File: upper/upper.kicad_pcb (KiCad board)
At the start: 2 copper layers, 127 x 50.8 mm, 1 part, among them U1 RaspberryPi_Pico_W

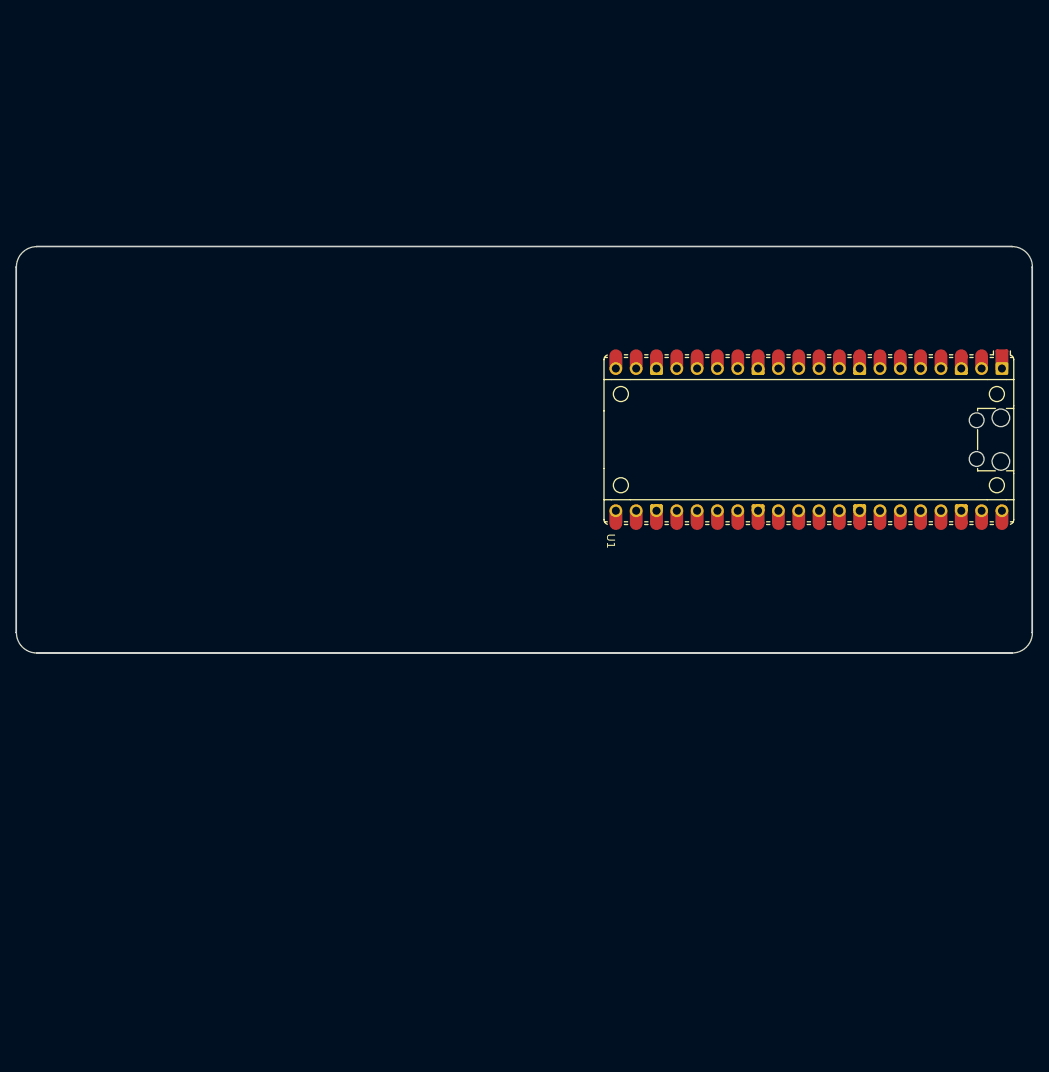
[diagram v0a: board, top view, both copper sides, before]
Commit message: Upper v0.0.1. Pre-routed
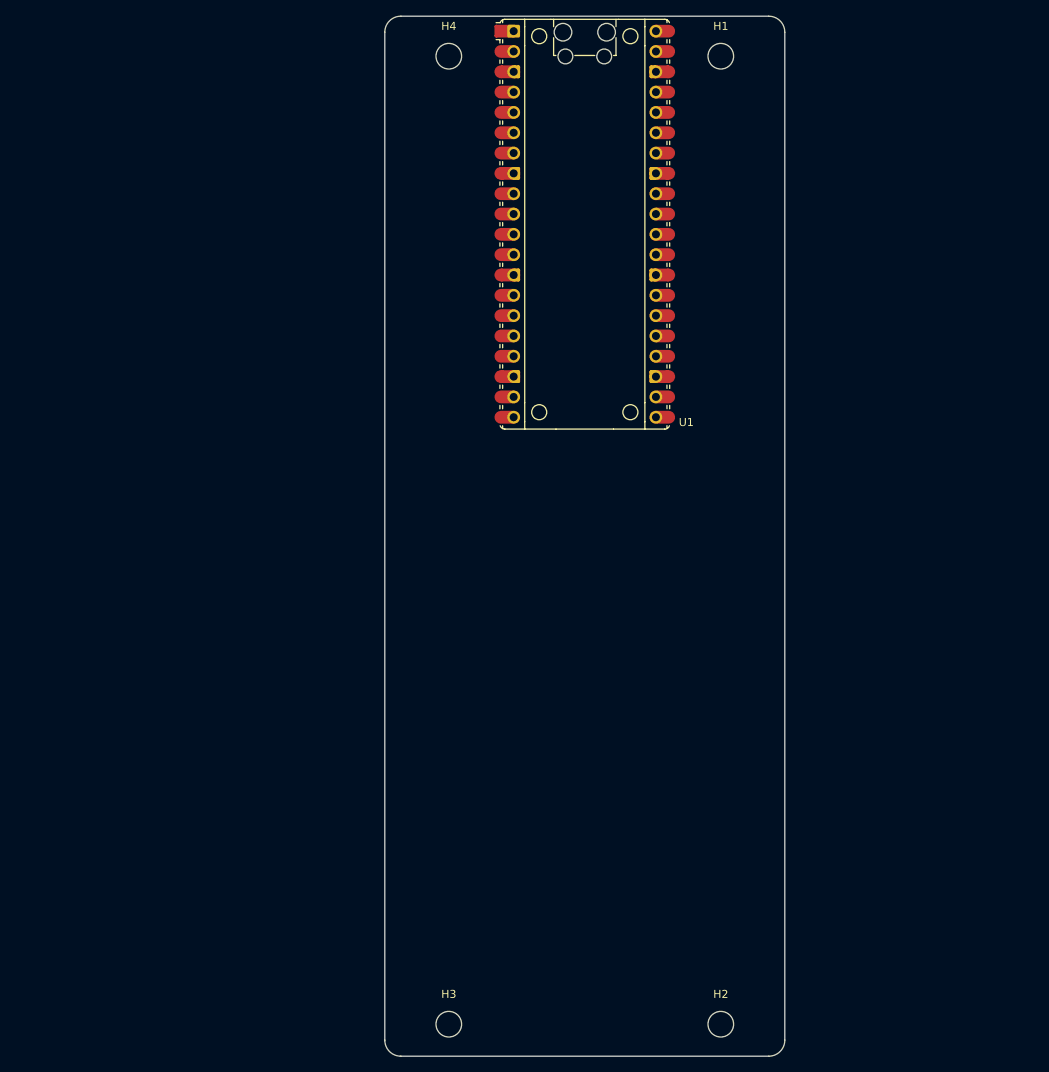
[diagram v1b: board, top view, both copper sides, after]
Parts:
- added H1: MountingHole, MountingHole:MountingHole_3.2mm_M3_ISO14580, F.Cu at (164.2, 27.0)
- added H2: MountingHole, MountingHole:MountingHole_3.2mm_M3_ISO14580, F.Cu at (164.2, 148.0)
- added H3: MountingHole, MountingHole:MountingHole_3.2mm_M3_ISO14580, F.Cu at (130.2, 148.0)
- added H4: MountingHole, MountingHole:MountingHole_3.2mm_M3_ISO14580, F.Cu at (130.2, 27.0)
- moved U1 38.9 mm to (147.2, 48.0), turned to 0 degrees
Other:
- board size 127 x 50.8 mm -> 50 x 130 mm
